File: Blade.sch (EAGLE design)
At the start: 168 parts, among them IC1 THN10-2411WIR, IC10 MCP6064-E/SL, IC12 LM78L05ACMX/NOPB, IC13 CH340G, IC2 MCP6064-E/SL, IC3 MCP6064-E/SL, IC4 MCP6064-E/SL, IC5 MAX488CSA, IC6 MOCD207MSOIC-8, IC7 MOCD207MSOIC-8, IC8 MOCD207MSOIC-8, IC9 MCP6064-E/SL, Q1 12MHz, U1 ADR366WAUJZ, U10 ADS1148QPWRQ1, U11 ADS1148QPWRQ1, U12 ADS1148QPWRQ1, U13 ADR366WAUJZ, U2 ADR366WAUJZ, U3 ADS1148QPWRQ1, U4 ADS1148QPWRQ1, U5 ADS1148QPWRQ1, U6 LT1528, U7 S70FL01GS, U8 S70FL01GS, U9 STM32F77XXXLQFP208, X1 D-SUB9-H5M09RA, X2 D-SUB15-H5M15RA, X3 USBPTH

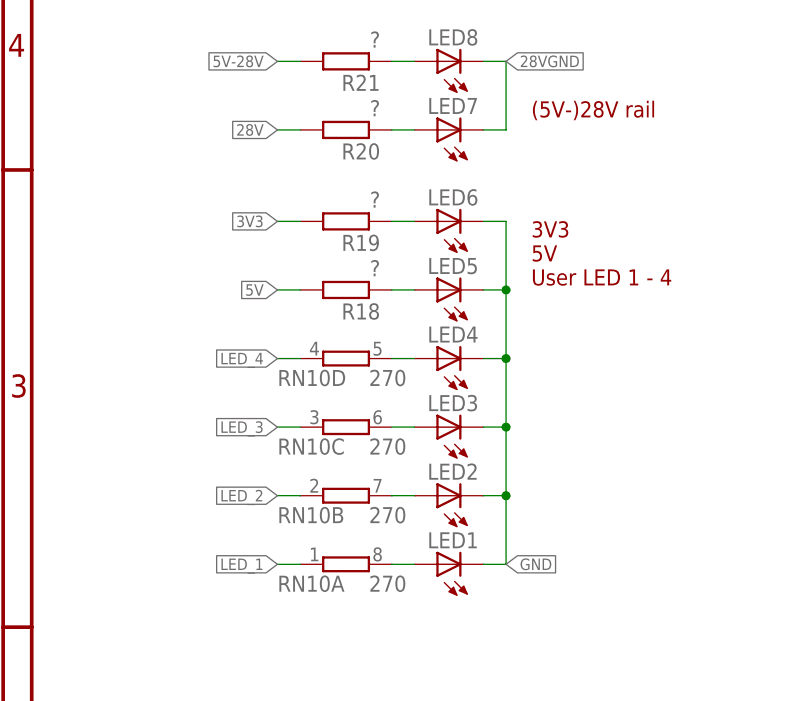
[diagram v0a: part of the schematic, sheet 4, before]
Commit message: Werte Update
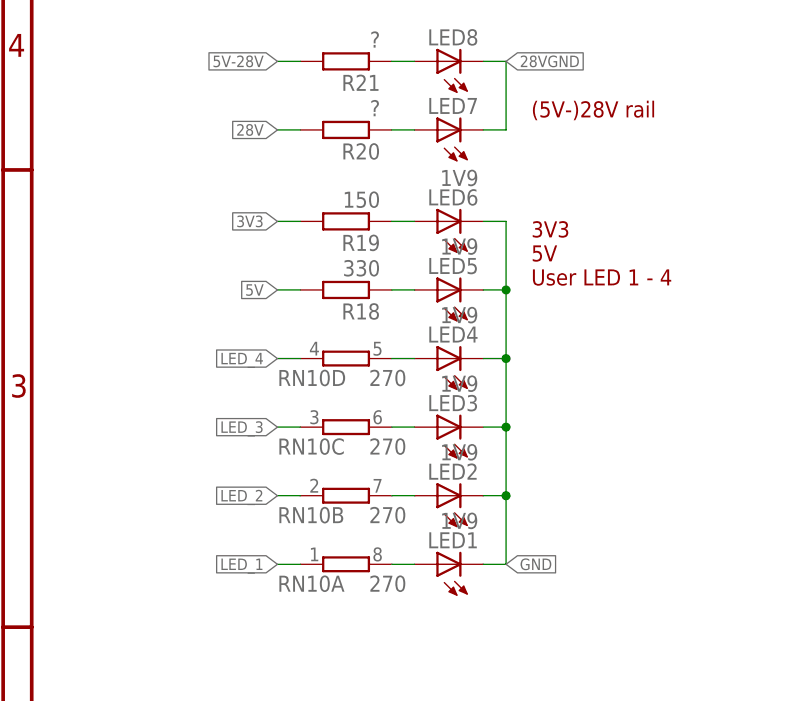
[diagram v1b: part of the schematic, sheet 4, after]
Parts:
- LED1, LED2, LED3, LED4, LED5, LED6: value (none) -> 1V9
- R18: value ? -> 330
- R19: value ? -> 150
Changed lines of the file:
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@@
 <?xml version="1.0" encoding="utf-8"?>
 <!DOCTYPE eagle SYSTEM "eagle.dtd">
-<eagle version="9.6.0">
+<eagle version="9.3.1">
 <drawing>
 <settings>
-<setting alwaysvectorfont="no"/>
+<setting alwaysvectorfont="yes"/>
 <setting verticaltext="up"/>
 </settings>
@@
 <part name="C14" library="rcl" library_urn="urn:adsk.eagle:library:334" deviceset="C-EU" device="C0805" package3d_urn="urn:adsk.eagle:package:23617/2" value="10u"/>
 <part name="C15" library="rcl" library_urn="urn:adsk.eagle:library:334" deviceset="CPOL-EU" device="153CLV-0810" package3d_urn="urn:adsk.eagle:package:23401/2" value="10u"/>
-<part name="LED1" library="adafruit" library_urn="urn:adsk.eagle:library:420" deviceset="LED" device="CHIP-LED0603" package3d_urn="urn:adsk.eagle:package:6240556/1"/>
-<part name="LED2" library="adafruit" library_urn="urn:adsk.eagle:library:420" deviceset="LED" device="CHIP-LED0603" package3d_urn="urn:adsk.eagle:package:6240556/1"/>
-<part name="LED3" library="adafruit" library_urn="urn:adsk.eagle:library:420" deviceset="LED" device="CHIP-LED0603" package3d_urn="urn:adsk.eagle:package:6240556/1"/>
-<part name="LED4" library="adafruit" library_urn="urn:adsk.eagle:library:420" deviceset="LED" device="CHIP-LED0603" package3d_urn="urn:adsk.eagle:package:6240556/1"/>
+<part name="LED1" library="adafruit" library_urn="urn:adsk.eagle:library:420" deviceset="LED" device="CHIP-LED0603" package3d_urn="urn:adsk.eagle:package:6240556/1" value="1V9"/>
+<part name="LED2" library="adafruit" library_urn="urn:adsk.eagle:library:420" deviceset="LED" device="CHIP-LED0603" package3d_urn="urn:adsk.eagle:package:6240556/1" value="1V9"/>
+<part name="LED3" library="adafruit" library_urn="urn:adsk.eagle:library:420" deviceset="LED" device="CHIP-LED0603" package3d_urn="urn:adsk.eagle:package:6240556/1" value="1V9"/>
+<part name="LED4" library="adafruit" library_urn="urn:adsk.eagle:library:420" deviceset="LED" device="CHIP-LED0603" package3d_urn="urn:adsk.eagle:package:6240556/1" value="1V9"/>
 <part name="RN10" library="resistor-dil" library_urn="urn:adsk.eagle:library:342" deviceset="4R-N" device="EXBS8V" package3d_urn="urn:adsk.eagle:package:24925/1" value="270"/>
 <part name="C16" library="rcl" library_urn="urn:adsk.eagle:library:334" deviceset="C-EU" device="C1206" package3d_urn="urn:adsk.eagle:package:23618/2" value="2.2u"/>
@@
 <part name="R16" library="rcl" deviceset="R-EU_" device="R0805" value="3k3"/>
 <part name="R17" library="rcl" deviceset="R-EU_" device="R0805" value="3k3"/>
-<part name="LED5" library="adafruit" library_urn="urn:adsk.eagle:library:420" deviceset="LED" device="CHIP-LED0603" package3d_urn="urn:adsk.eagle:package:6240556/1"/>
-<part name="LED6" library="adafruit" library_urn="urn:adsk.eagle:library:420" deviceset="LED" device="CHIP-LED0603" package3d_urn="urn:adsk.eagle:package:6240556/1"/>
-<part name="R18" library="rcl" library_urn="urn:adsk.eagle:library:334" deviceset="R-EU_" device="R0805" package3d_urn="urn:adsk.eagle:package:23553/2" value="?"/>
-<part name="R19" library="rcl" library_urn="urn:adsk.eagle:library:334" deviceset="R-EU_" device="R0805" package3d_urn="urn:adsk.eagle:package:23553/2" value="?"/>
+<part name="LED5" library="adafruit" library_urn="urn:adsk.eagle:library:420" deviceset="LED" device="CHIP-LED0603" package3d_urn="urn:adsk.eagle:package:6240556/1" value="1V9"/>
+<part name="LED6" library="adafruit" library_urn="urn:adsk.eagle:library:420" deviceset="LED" device="CHIP-LED0603" package3d_urn="urn:adsk.eagle:package:6240556/1" value="1V9"/>
+<part name="R18" library="rcl" library_urn="urn:adsk.eagle:library:334" deviceset="R-EU_" device="R0805" package3d_urn="urn:adsk.eagle:package:23553/2" value="330"/>
+<part name="R19" library="rcl" library_urn="urn:adsk.eagle:library:334" deviceset="R-EU_" device="R0805" package3d_urn="urn:adsk.eagle:package:23553/2" value="150"/>
 <part name="LED7" library="adafruit" library_urn="urn:adsk.eagle:library:420" deviceset="LED" device="CHIP-LED0603" package3d_urn="urn:adsk.eagle:package:6240556/1"/>
 <part name="R20" library="rcl" library_urn="urn:adsk.eagle:library:334" deviceset="R-EU_" device="R0805" package3d_urn="urn:adsk.eagle:package:23553/2" value="?"/>
